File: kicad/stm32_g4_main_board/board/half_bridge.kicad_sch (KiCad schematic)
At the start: 4 parts, among them Q1 CSD18514Q5A, Q2 CSD18514Q5A

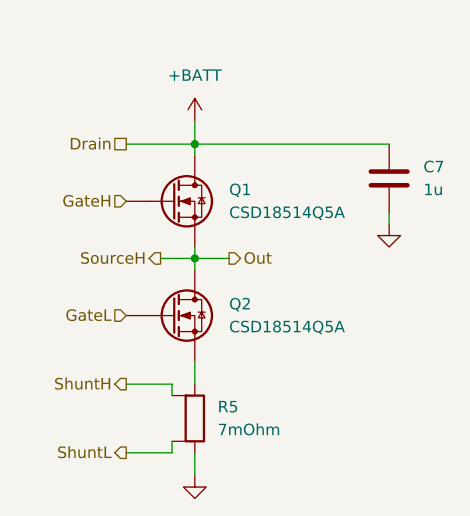
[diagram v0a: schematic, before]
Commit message: WIP - v2 board
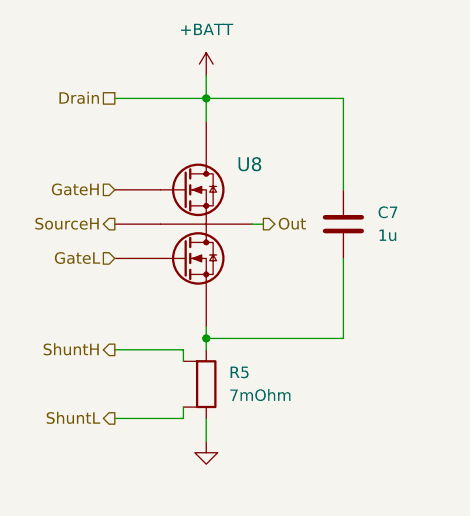
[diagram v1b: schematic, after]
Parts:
- removed Q1, Q2: CSD18514Q5A, jaguilar:CSD18514Q5A, symbol jaguilar:CSD18514Q5A
- added U8: CSD88584Q5DC, jaguilar:DMM0022A, symbol jaguilar:CSD88584Q5DC
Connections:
- net +BATT: now also U8.27 (VIN)
- net GND: no longer C7.1
- net GateH: now also U8.1 (GH)
- net GateL: now also U8.22 (GL)
- net Out: now also U8.[3,4,5,6,7,8,9,10,11] (VSW)
- net at R5.1: now also C7.1, U8.[12,13,14,15,16,17,18,19,20] (PGND)
- new net: U8.21 (NC), U8.23 (NC), U8.24 (NC), U8.25 (NC), U8.26 (NC)
- new net SourceH: U8.2 (SH)
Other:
- moved on the sheet: C7, R5
